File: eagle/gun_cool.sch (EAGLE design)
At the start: 19 parts, among them IC2 AD823, IC3 LM358

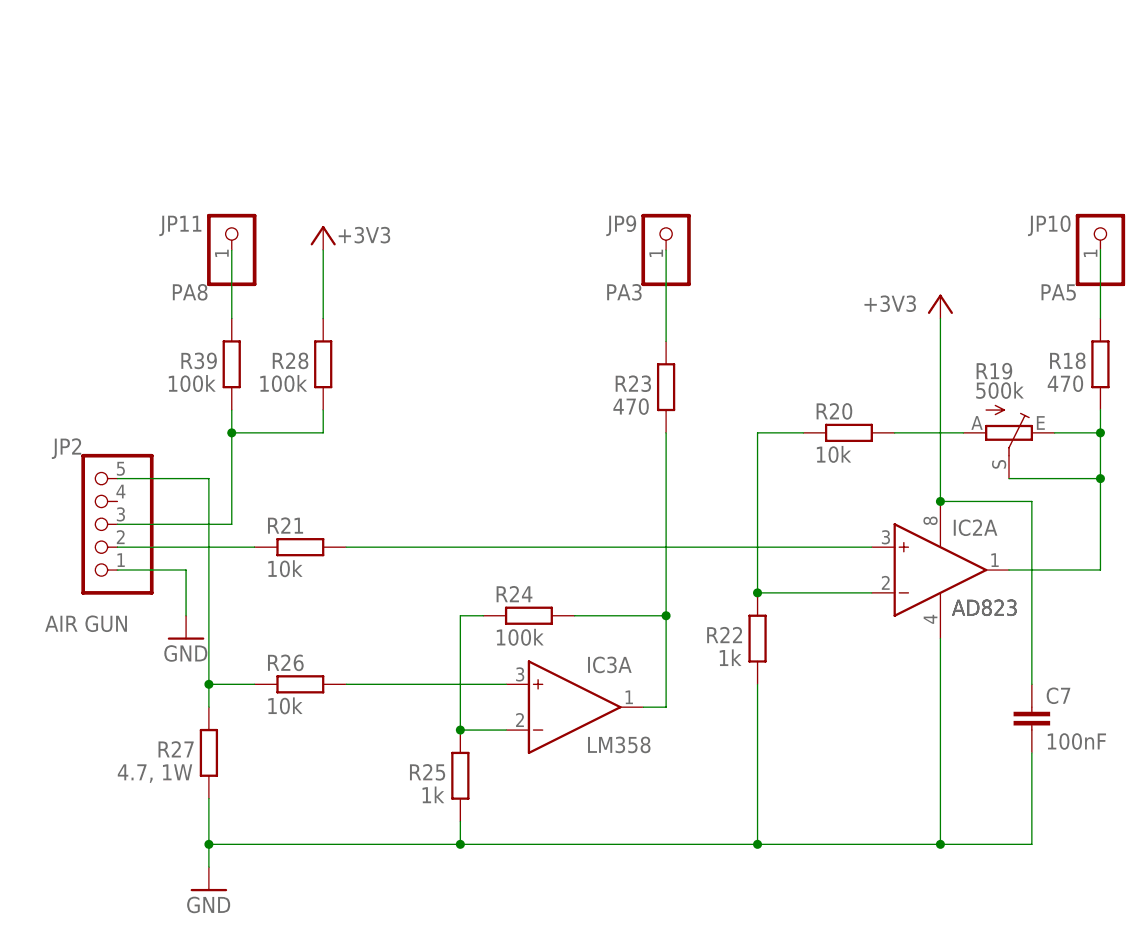
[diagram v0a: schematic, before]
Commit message: Add files via upload
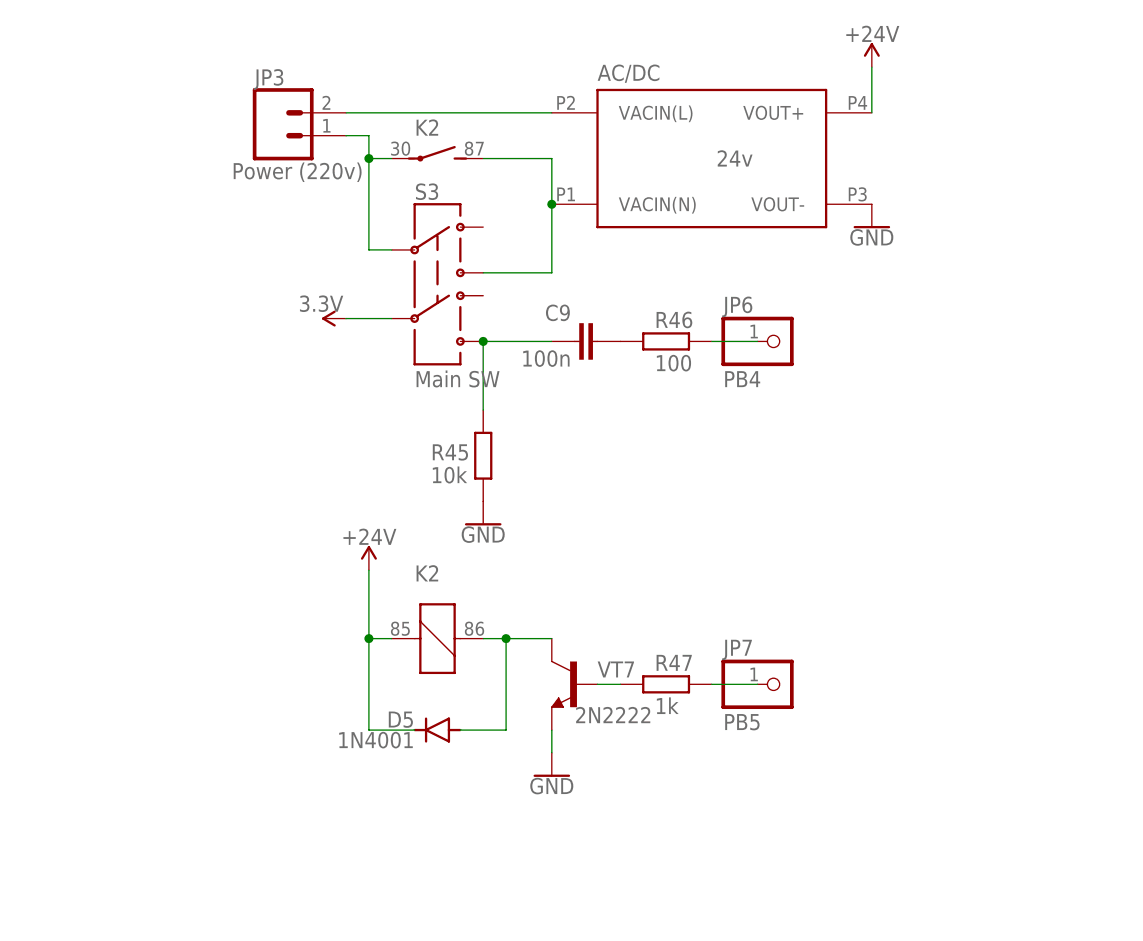
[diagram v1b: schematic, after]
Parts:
- removed C7: 100nF, rcl:C-EU025-024X044
- removed IC2: AD823, analog-devices:AD822N
- removed IC3: LM358, analog-devices:AD822N
- removed JP10: PA5, pinhead:PINHD-1X1
- removed JP11: PA8, pinhead:PINHD-1X1
- removed JP2: AIR GUN, pinhead:PINHD-1X5
- removed JP9: PA3, pinhead:PINHD-1X1
- removed R18, R23: 470, rcl:R-EU_0204/5
- removed R19: 500k, pot:TRIM_EU-B64Y
- removed R20, R21, R26: 10k, rcl:R-EU_0204/5
- removed R22, R25: 1k, rcl:R-EU_0204/5
- removed R24, R28, R39: 100k, rcl:R-EU_0204/5
- removed R27: 4.7, 1W, rcl:R-EU_0204/5
- added AC/DC: 24v, recom-powerline-acdc-converters:RAC02-24SC
- added C9: 100n, rcl:C-EUC1206
- added D5: 1N4001, diode:1N4004
- added JP3: Power (220v), SparkFun-Connectors:CONN_02
- added JP6: PB4, pinhead:PINHD-1X1
- added JP7: PB5, pinhead:PINHD-1X1
- added K2: CB1A-T-P-24V, relay:CB1A-T-P-24V
- added R45: 10k, rcl:R-EU_M1206
- added R46: 100, rcl:R-EU_M1206
- added R47: 1k, rcl:R-EU_M1206
- added S3: Main SW, SparkFun-Retired:SWITCH-DPDTOS
- added VT7: 2N2222, transistor:2N2222
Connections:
- removed net +3V3: C7.1, IC2P.V+, R28.2
- removed net N$10: R19.A, R20.2
- removed net N$11: IC2A.OUT, R18.1, R19.E, R19.S
- removed net N$12: IC2A.IN-, R20.1, R22.2
- removed net N$13: JP11.1, R39.2
- new net 3.3V: S3.5
- new net VCC: AC/DC.VOUT+, D5.C, K21.2
- net GND: now also AC/DC.VOUT-, R45.1, VT7.E; no longer C7.2, IC2P.V-, JP2.1, R22.1, R25.1, R27.1
- net N$1: now also AC/DC.VACIN(L), JP3.2; no longer JP2.5, R26.1, R27.2
- net N$2: now also JP3.1, K22.P, S3.2; no longer IC3A.IN+, R26.2
- net N$3: now also AC/DC.VACIN(N), K22.S, S3.3; no longer IC3A.IN-, R24.1, R25.2
- net N$4: now also C9.1, R45.2, S3.6; no longer IC3A.OUT, R23.1, R24.2
- net N$5: now also C9.2, R46.1; no longer IC2A.IN+, R21.2
- net N$6: now also JP6.1, R46.2; no longer JP2.2, R21.1
- net N$7: now also JP7.1, R47.2; no longer JP2.3, R28.1, R39.1
- net N$8: now also R47.1, VT7.B; no longer JP9.1, R23.2
- net N$9: now also D5.A, K21.1, VT7.C; no longer JP10.1, R18.2
